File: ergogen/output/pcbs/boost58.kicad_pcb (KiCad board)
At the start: 2 copper layers, 147.8 x 127.7 mm, 110 parts, among them SW1 ${REFERENCE}, SW10 ${REFERENCE}, SW11 ${REFERENCE}, SW12 ${REFERENCE}, SW13 ${REFERENCE}, SW14 ${REFERENCE}, SW15 ${REFERENCE}, SW16 ${REFERENCE}, SW17 ${REFERENCE}, SW18 ${REFERENCE}, SW19 ${REFERENCE}, SW2 ${REFERENCE}, SW20 ${REFERENCE}, SW21 ${REFERENCE}, SW22 ${REFERENCE}, SW23 ${REFERENCE}, SW24 ${REFERENCE}, SW25 ${REFERENCE}, SW26 ${REFERENCE}, SW27 ${REFERENCE}, SW28 ${REFERENCE}, SW29 ${REFERENCE}, SW3 ${REFERENCE}, SW4 ${REFERENCE}, SW5 ${REFERENCE}, SW6 ${REFERENCE}, SW7 ${REFERENCE}, SW8 ${REFERENCE}, SW9 ${REFERENCE}

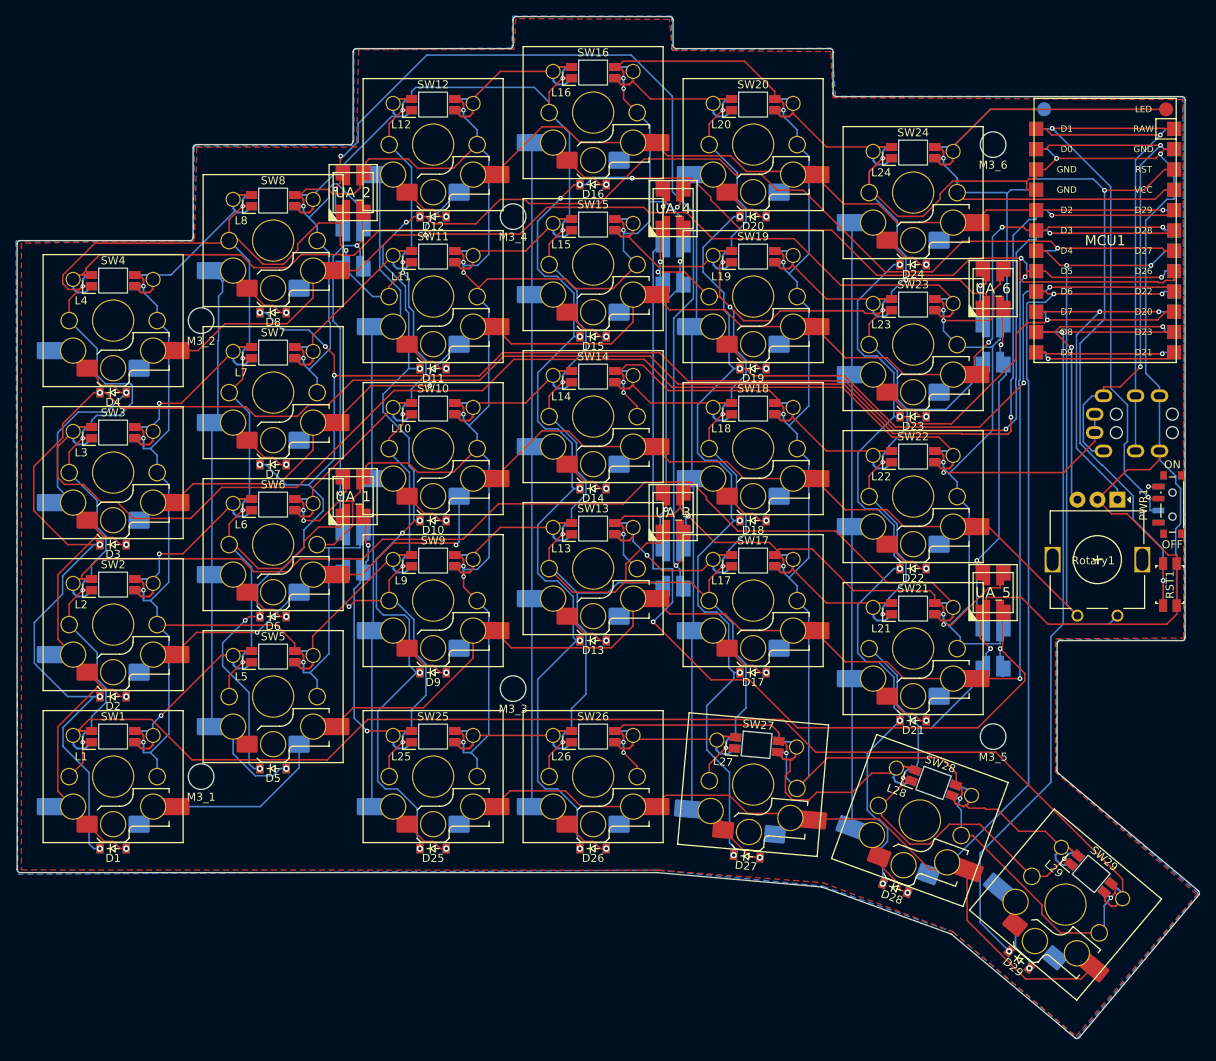
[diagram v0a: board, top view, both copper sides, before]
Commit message: re-generated pcb's and outlines
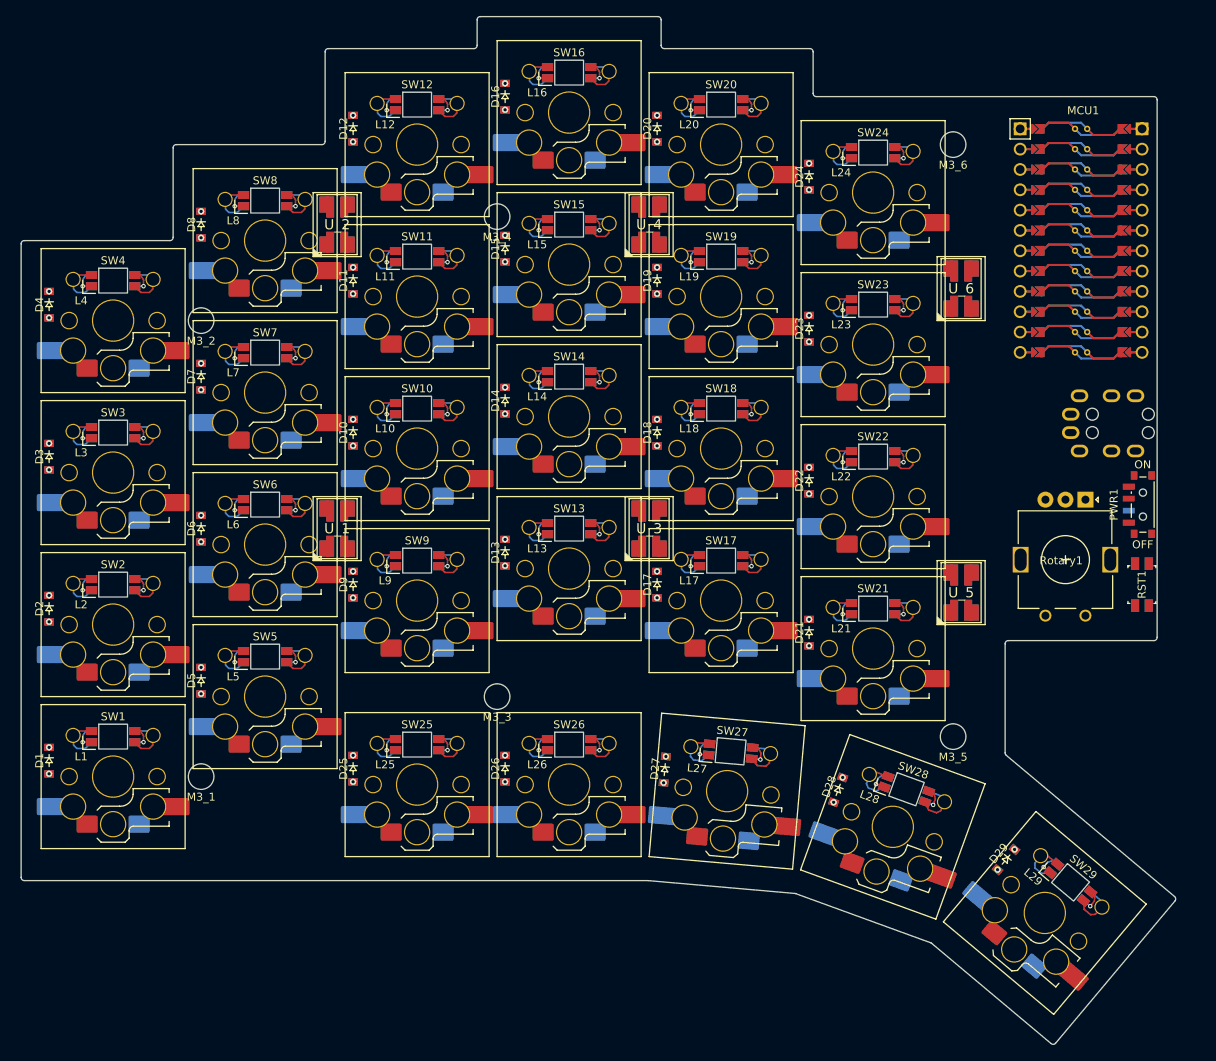
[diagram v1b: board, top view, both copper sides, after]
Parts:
- removed UA_1, UA_2, UA_3, UA_4, UA_5, UA_6, UB_1, UB_2, UB_3, UB_4, UB_5, UB_6: , WS2812B
- added U_1: , WS2812B, F.Cu at (68.0, 89.0)
- added U_2: , WS2812B, F.Cu at (68.0, 51.0)
- added U_3: , WS2812B, F.Cu at (107.0, 89.0)
- added U_4: , WS2812B, F.Cu at (107.0, 51.0)
- added U_5: , WS2812B, F.Cu at (146.0, 97.0)
- added U_6: , WS2812B, F.Cu at (146.0, 59.0)
- D1, D10, D11, D12, D13, D14, D15, D16, D17, D18, D19, D2, D20, D21, D22, D23, D24, D25, D26, D27, D28, D29, D3, D4, D5, D6, D7, D8, D9, L1, L10, L11, L12, L13, L14, L15, L16, L17, L18, L19, L2, L20, L21, L22, L23, L24, L25, L26, L27, L28, L29, L3, L4, L5, L6, L7, L8, L9, SW1, SW10, SW11, SW12, SW13, SW14, SW15, SW16, SW17, SW18, SW19, SW2, SW20, SW21, SW22, SW23, SW24, SW25, SW26, SW27, SW28, SW29, SW3, SW4, SW5, SW6, SW7, SW8, SW9: value ${REFERENCE} -> %R
- MCU1: footprint SparkFunProMicroQwiic -> ProMicro
- moved D21 17.0 mm to (127.0, 102.0), turned to -90 degrees
- moved D22 17.0 mm to (127.0, 83.0), turned to -90 degrees
- moved D23 17.0 mm to (127.0, 64.0), turned to -90 degrees
- moved D24 17.0 mm to (127.0, 45.0), turned to -90 degrees
- moved D17 16.3 mm to (108.0, 96.0), turned to -90 degrees
- moved D18 16.3 mm to (108.0, 77.0), turned to -90 degrees
- moved D19 16.3 mm to (108.0, 58.0), turned to -90 degrees
- moved D20 16.3 mm to (108.0, 39.0), turned to -90 degrees
- moved D13 15.6 mm to (89.0, 92.0), turned to -90 degrees
- moved D14 15.6 mm to (89.0, 73.0), turned to -90 degrees
- moved D15 15.6 mm to (89.0, 54.0), turned to -90 degrees
- moved D16 15.6 mm to (89.0, 35.0), turned to -90 degrees
- moved D27 14.9 mm to (109.0, 119.1), turned to -95 degrees
- moved D10 14.9 mm to (70.0, 77.0), turned to -90 degrees
- moved D11 14.9 mm to (70.0, 58.0), turned to -90 degrees
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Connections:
- D1 pad 1: D29 -> P21
- D1 pad 2: DD29 -> DP21
- D10 pad 1: D27 -> P19
- D10 pad 2: DD27 -> DP19
- D11 pad 1: D27 -> P19
- D11 pad 2: DD27 -> DP19
- D12 pad 1: D27 -> P19
- D12 pad 2: DD27 -> DP19
- D13 pad 1: D26 -> P18
- D13 pad 2: DD26 -> DP18
- D14 pad 1: D26 -> P18
- D14 pad 2: DD26 -> DP18
- D15 pad 1: D26 -> P18
- D15 pad 2: DD26 -> DP18
- D16 pad 1: D26 -> P18
- D16 pad 2: DD26 -> DP18
- D17 pad 1: D22 -> P15
- D17 pad 2: DD22 -> DP15
- D18 pad 1: D22 -> P15
- D18 pad 2: DD22 -> DP15
- D19 pad 1: D22 -> P15
- D19 pad 2: DD22 -> DP15
- D2 pad 1: D29 -> P21
- D2 pad 2: DD29 -> DP21
- D20 pad 1: D22 -> P15
- D20 pad 2: DD22 -> DP15
- D21 pad 1: D20 -> P14
- D21 pad 2: DD20 -> DP14
- D22 pad 1: D20 -> P14
- D22 pad 2: DD20 -> DP14
- D23 pad 1: D20 -> P14
- D23 pad 2: DD20 -> DP14
- D24 pad 1: D20 -> P14
- D24 pad 2: DD20 -> DP14
- D25 pad 1: D27 -> P21
- D25 pad 2: DD27 -> DP21
- D26 pad 1: D26 -> P20
- D26 pad 2: DD26 -> DP20
- D27 pad 1: D22 -> P19
- D27 pad 2: DD22 -> DP19
- D28 pad 1: D20 -> P18
- D28 pad 2: DD20 -> DP18
- D29 pad 1: D23 -> P15
- D29 pad 2: DD23 -> DP15
- D3 pad 1: D29 -> P21
- D3 pad 2: DD29 -> DP21
- D4 pad 1: D29 -> P21
- D4 pad 2: DD29 -> DP21
- D5 pad 1: D28 -> P20
- D5 pad 2: DD28 -> DP20
- D6 pad 1: D28 -> P20
- D6 pad 2: DD28 -> DP20
- D7 pad 1: D28 -> P20
- D7 pad 2: DD28 -> DP20
- D8 pad 1: D28 -> P20
- D8 pad 2: DD28 -> DP20
- D9 pad 1: D27 -> P19
- D9 pad 2: DD27 -> DP19
- MCU1 pad 1: D1 -> RAW
- MCU1 pad 2: D2 -> GND
- MCU1 pad 20: D20 -> P2
- MCU1 pad 21: D21 -> GND
- MCU1 pad 22: D22 -> GND
- MCU1 pad 23: D23 -> P0
- MCU1 pad 3: D3 -> RST
- MCU1 pad 4: D4 -> VCC
- MCU1 pad 5: D5 -> P21
- MCU1 pad 6: D6 -> P20
- MCU1 pad 7: D7 -> P19
- MCU1 pad 8: D8 -> P18
- MCU1 pad 9: D9 -> P15
- Rotary1 pad 1: D23 -> P14
- Rotary1 pad 2: D4 -> P6
- Rotary1 pad A: D7 -> P7
- Rotary1 pad B: D8 -> P8
- SW1 pad : GND -> LED11
- SW1 pad 1: D5 -> P5
- SW1 pad 2: DD29 -> DP21
- SW10 pad : GND -> LED23
- SW10 pad 1: D4 -> P4
- SW10 pad 2: DD27 -> DP19
- SW11 pad : GND -> LED33
- SW11 pad 1: D3 -> P3
- SW11 pad 2: DD27 -> DP19
- SW12 pad : GND -> LED43
- SW12 pad 1: D2 -> P2
- SW12 pad 2: DD27 -> DP19
- SW13 pad : GND -> LED14
- SW13 pad 1: D5 -> P5
- SW13 pad 2: DD26 -> DP18
- SW14 pad : GND -> LED24
- SW14 pad 1: D4 -> P4
- SW14 pad 2: DD26 -> DP18
- SW15 pad : GND -> LED34
- SW15 pad 1: D3 -> P3
- SW15 pad 2: DD26 -> DP18
- SW16 pad : GND -> LED44
- SW16 pad 1: D2 -> P2
- SW16 pad 2: DD26 -> DP18
- SW17 pad : GND -> LED15
- SW17 pad 1: D5 -> P5
- SW17 pad 2: DD22 -> DP15
- SW18 pad : GND -> LED25
- SW18 pad 1: D4 -> P4
- SW18 pad 2: DD22 -> DP15
- SW19 pad : GND -> LED35
- SW19 pad 1: D3 -> P3
- SW19 pad 2: DD22 -> DP15
- SW2 pad : GND -> LED21
- SW2 pad 1: D4 -> P4
- SW2 pad 2: DD29 -> DP21
- SW20 pad : GND -> LED45
- SW20 pad 1: D2 -> P2
- SW20 pad 2: DD22 -> DP15
- SW21 pad : GND -> LED20
- SW21 pad 1: D5 -> P5
- SW21 pad 2: DD20 -> DP14
- SW22 pad : GND -> LED30
- SW22 pad 1: D4 -> P4
- SW22 pad 2: DD20 -> DP14
- SW23 pad : GND -> LED40
- SW23 pad 1: D3 -> P3
- SW23 pad 2: DD20 -> DP14
- SW24 pad : GND -> LED
- SW24 pad 1: D2 -> P2
- SW24 pad 2: DD20 -> DP14
- SW25 pad : GND -> LED02
- SW25 pad 1: D6 -> P6
- SW25 pad 2: DD27 -> DP21
- SW26 pad : GND -> LED03
- SW26 pad 1: D6 -> P6
- SW26 pad 2: DD26 -> DP20
- SW27 pad : GND -> LED04
- SW27 pad 1: D6 -> P6
- SW27 pad 2: DD22 -> DP19
- SW28 pad : GND -> LED05
- SW28 pad 1: D6 -> P6
- SW28 pad 2: DD20 -> DP18
- SW29 pad : GND -> LED10
- SW29 pad 1: D6 -> P6
- SW29 pad 2: DD23 -> DP15
- SW3 pad : GND -> LED31
- SW3 pad 1: D3 -> P3
- SW3 pad 2: DD29 -> DP21
- SW4 pad : GND -> LED41
- SW4 pad 1: D2 -> P2
- SW4 pad 2: DD29 -> DP21
- SW5 pad : GND -> LED12
- SW5 pad 1: D5 -> P5
- SW5 pad 2: DD28 -> DP20
- SW6 pad : GND -> LED22
- SW6 pad 1: D4 -> P4
- SW6 pad 2: DD28 -> DP20
- SW7 pad : GND -> LED32
- SW7 pad 1: D3 -> P3
- SW7 pad 2: DD28 -> DP20
- SW8 pad : GND -> LED42
- SW8 pad 1: D2 -> P2
- SW8 pad 2: DD28 -> DP20
- SW9 pad : GND -> LED13
- SW9 pad 1: D5 -> P5
- SW9 pad 2: DD27 -> DP19
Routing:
- net GND: track 1040.1 -> 96.3 mm, vias 39 -> 29
- net VCC: track 964.8 -> 96.3 mm, vias 40 -> 29
- net D29: track 249.3 -> 0.00 mm, vias 6 -> 0
- net D5: track 219.0 -> 0.00 mm, vias 3 -> 0
- net D4: track 215.6 -> 0.00 mm, vias 4 -> 0
- net D28: track 215.4 -> 0.00 mm, vias 9 -> 0
- net D27: track 208.9 -> 0.00 mm, vias 8 -> 0
- net D6: track 204.4 -> 0.00 mm, vias 2 -> 0
- net D26: track 192.9 -> 0.00 mm, vias 8 -> 0
- net D3: track 181.2 -> 0.00 mm, vias 4 -> 0
- net D22: track 169.4 -> 0.00 mm, vias 7 -> 0
- net D2: track 162.4 -> 0.00 mm, vias 2 -> 0
- net LED10: track 162.7 -> 13.5 mm
- net D20: track 142.2 -> 0.00 mm, vias 6 -> 0
- net DD26: track 141.7 -> 0.00 mm, vias 5 -> 0
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- removed copper zone on F.Cu, net GND
- removed copper zone on B.Cu, net VCC
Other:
- board size 147.8 x 127.7 mm -> 144.3 x 128.5 mm
